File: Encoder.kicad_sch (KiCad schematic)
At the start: 13 parts, among them J4 DE9_Socket, U2 AP3012, U3 AM26LS32ACDR, U4 AP2151AW-7

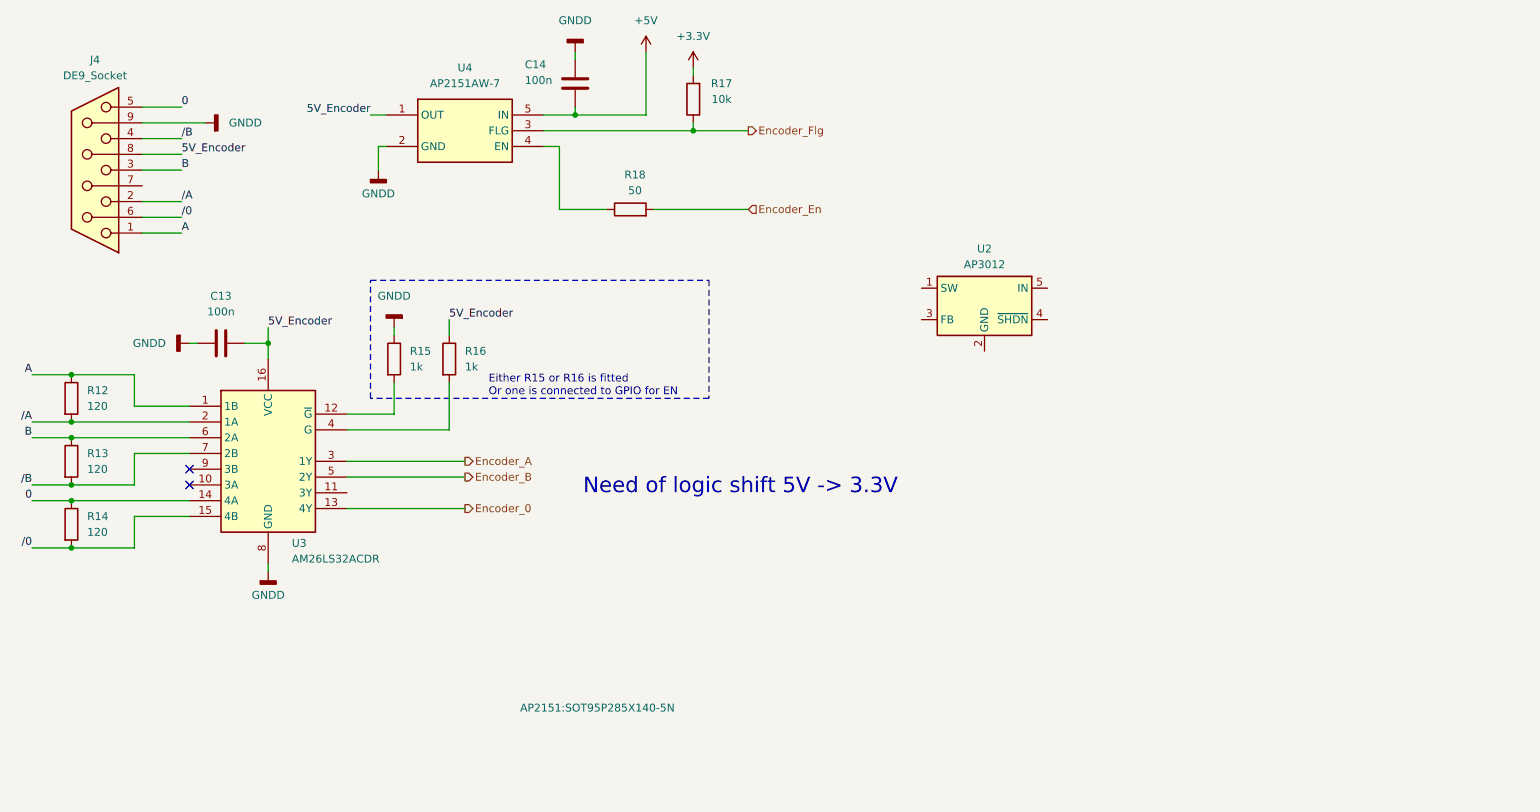
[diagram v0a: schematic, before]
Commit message: wip
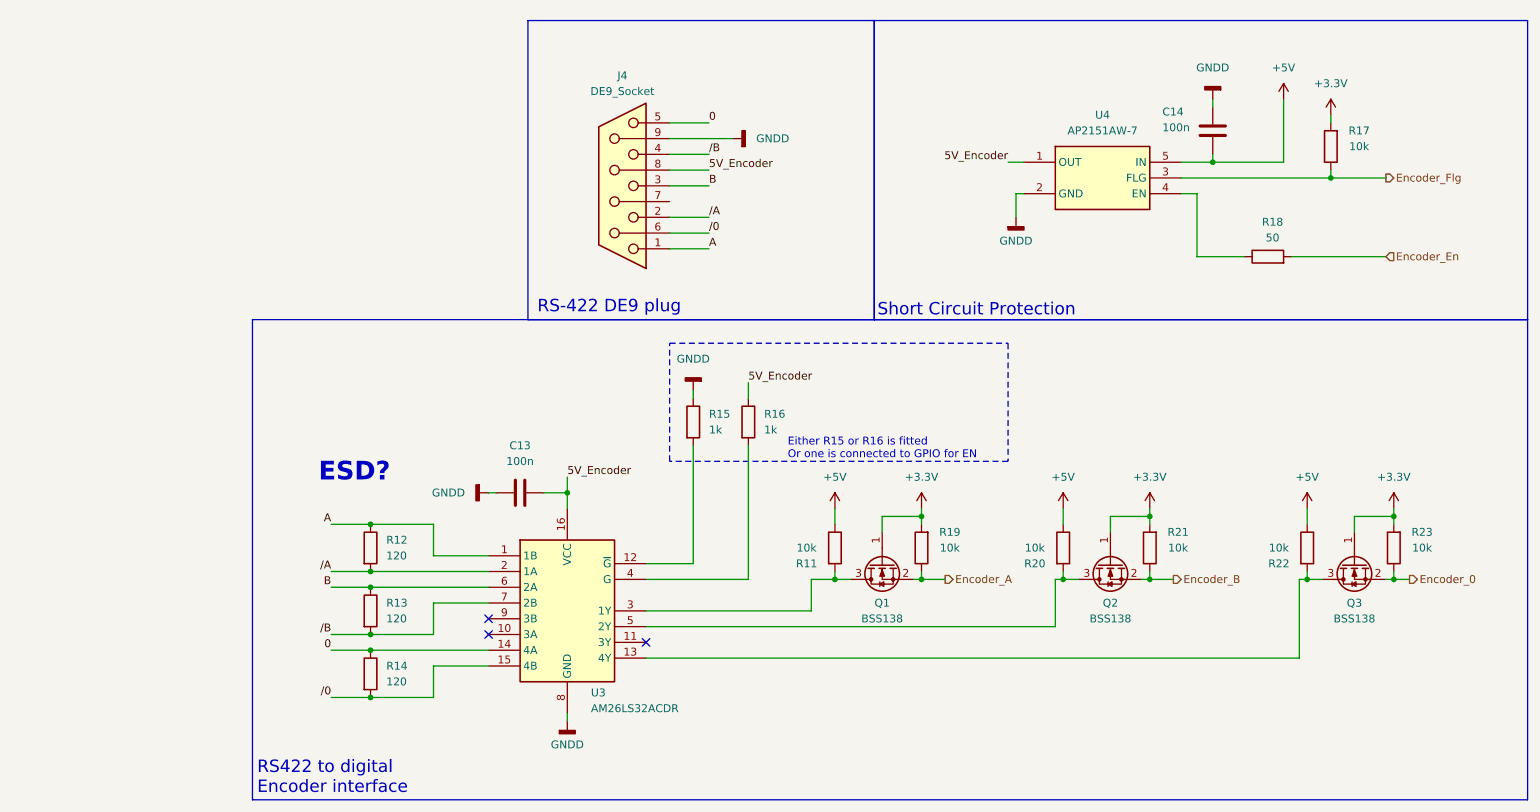
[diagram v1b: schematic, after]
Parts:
- removed U2: AP3012, Package_TO_SOT_SMD:SOT-23-5, symbol Regulator_Switching:AP3012
- added Q1, Q2, Q3: BSS138, Package_TO_SOT_SMD:SOT-23, symbol Transistor_FET:BSS138
- added R11, R19, R20, R21, R22, R23: 10k, Resistor_SMD:R_0805_2012Metric, symbol Device:R
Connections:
- net +3.3V: now also Q1.1 (G), Q2.1 (G), Q3.1 (G), R19.2, R21.2, R23.2
- net +5V: now also R11.1, R20.1, R22.1
- net Encoder_0: now also Q3.2 (S), R23.1; no longer U3.13 (4Y)
- net Encoder_A: now also Q1.2 (S), R19.1; no longer U3.3 (1Y)
- net Encoder_B: now also Q2.2 (S), R21.1; no longer U3.5 (2Y)
- new net: Q1.3 (D), R11.2, U3.3 (1Y)
- new net: Q3.3 (D), R22.2, U3.13 (4Y)
- new net: Q2.3 (D), R20.2, U3.5 (2Y)
- no-connect marks 2 -> 3
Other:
- note added: "ESD?"
- note added: "RS-422 DE9 plug"
- note added: "RS422 to digital Encoder interface"
- note added: "Short Circuit Protection"
- note removed: "Need of logic shift 5V -> 3.3V"
- moved on the sheet: C13, C14, J4, R12, R13, R14, R15, R16, R17, R18, U3, U4
